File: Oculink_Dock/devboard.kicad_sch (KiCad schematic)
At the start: 34 parts, among them J2 USB_C_Receptacle_USB2.0_14P, J5 Conn_01x10, J6 Conn_01x10, J7 Conn_01x10, J8 Conn_01x03, SW1 SW_Push, U1 RP2040, U2 NCP1117-3.3_SOT223, U3 W25Q128JVS, Y1 12 MHz

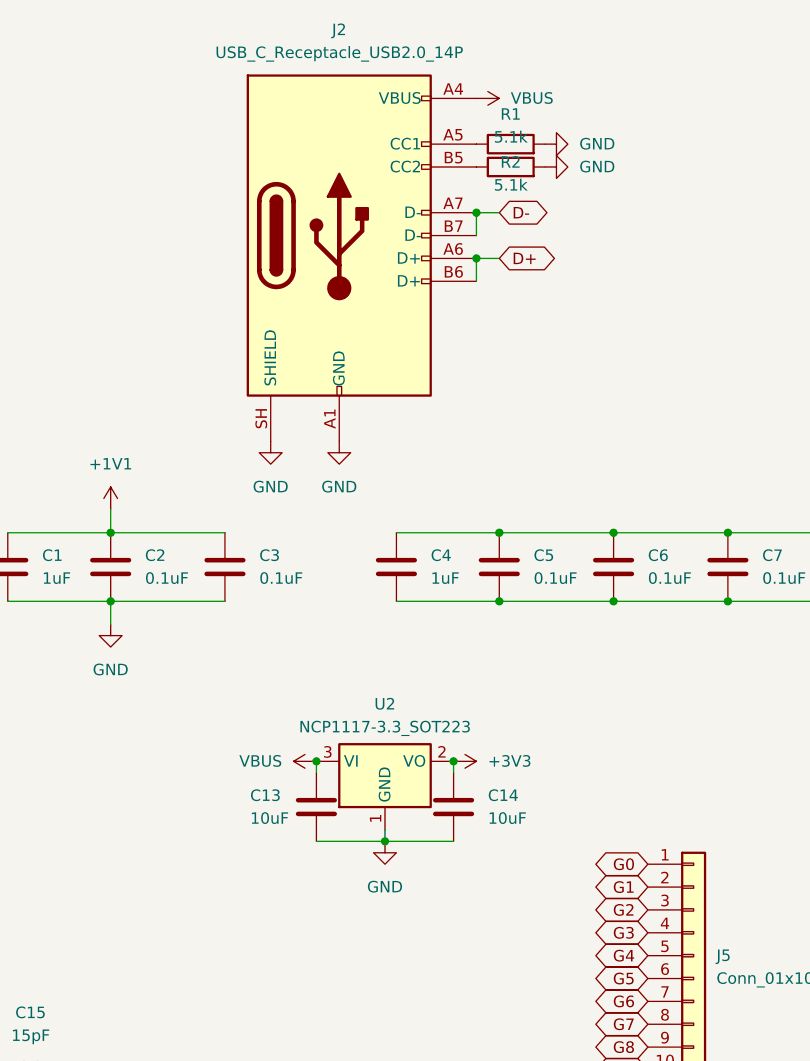
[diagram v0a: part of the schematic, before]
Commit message: Update
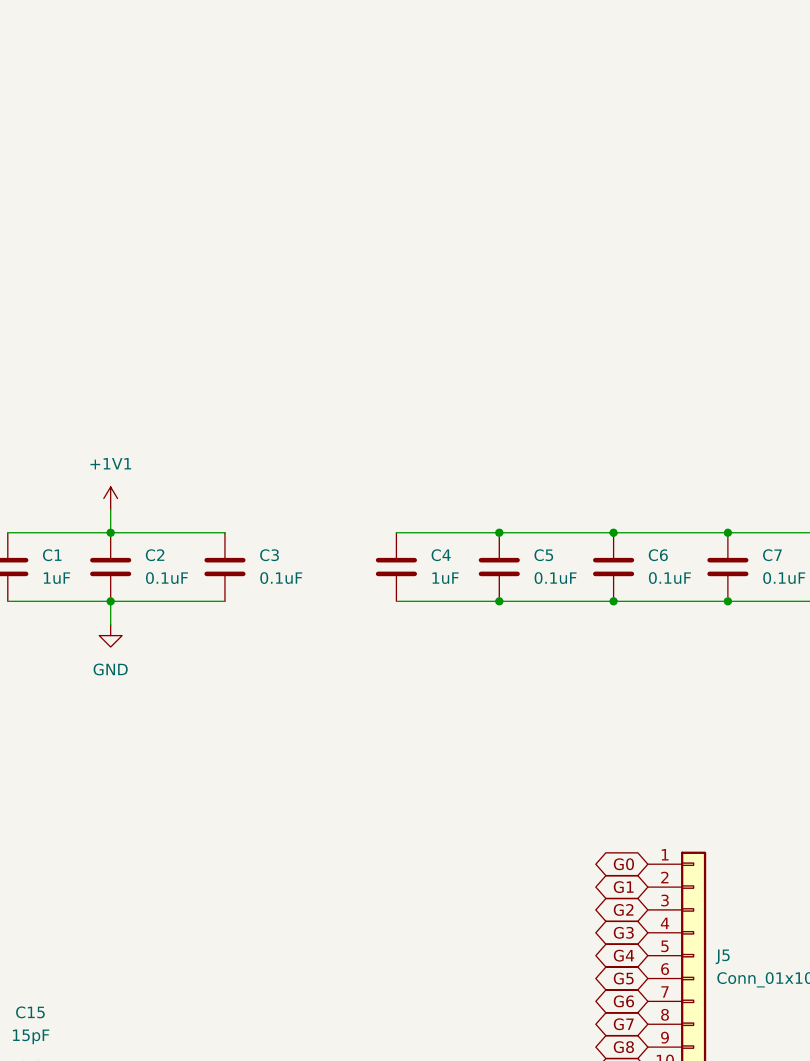
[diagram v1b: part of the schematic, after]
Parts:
- removed C13, C14: 10uF, symbol Device:C
- removed J2: USB_C_Receptacle_USB2.0_14P, Package_DFN_QFN:QFN-56-1EP_7x7mm_P0.4mm_EP3.2x3.2mm, symbol Connector:USB_C_Receptacle_USB2.0_14P
- removed R1, R2: 5.1k, symbol Device:R
- removed U2: NCP1117-3.3_SOT223, Package_TO_SOT_SMD:SOT-223-3_TabPin2, symbol Regulator_Linear:NCP1117-3.3_SOT223
